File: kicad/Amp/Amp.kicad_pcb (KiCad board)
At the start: 2 copper layers, 30 x 25.6 mm, 31 parts, among them J1 Conn, J2 Conn, J3 Conn, J4 Conn, J5 Conn, U1 TS5A3166DBVR, U2 MCP1700

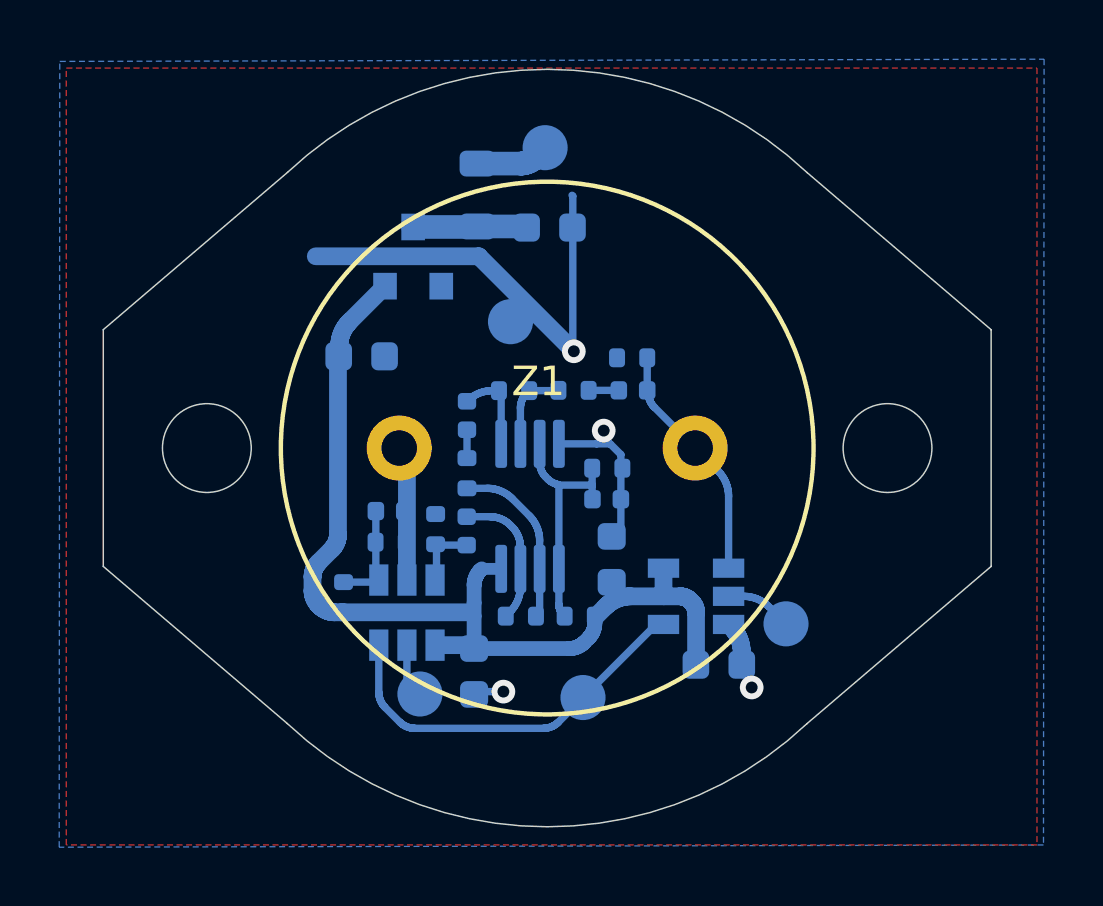
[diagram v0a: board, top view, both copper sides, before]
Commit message: изменено:      kicad/Amp/Amp.kicad_pcb 	изменено:      kicad/Amp/Amp.kicad_pcb-bak 	изменено:      kicad/Amp/Amp.sch 	изменено:      kicad/Amp/Amp.sch-bak 	изменено:      kicad/Amp/fp-info-cache
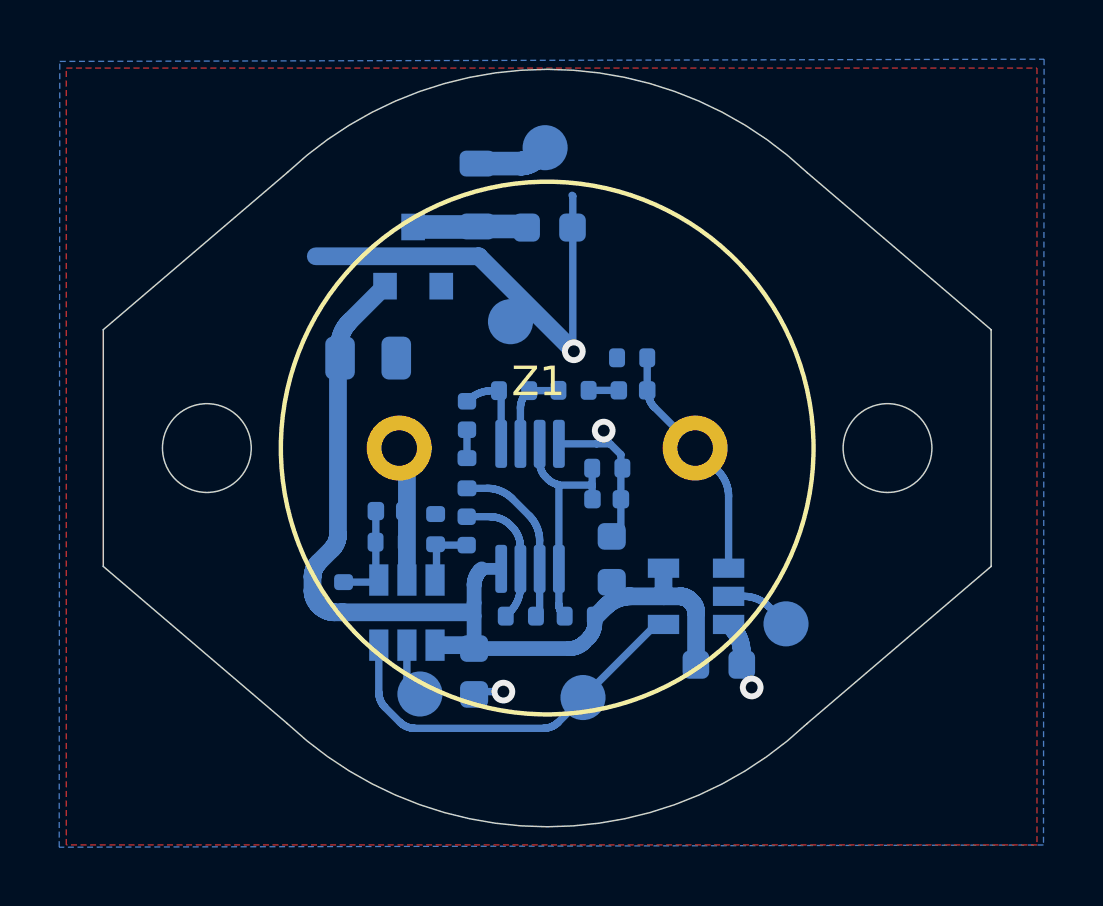
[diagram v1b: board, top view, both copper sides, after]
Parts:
- C5: value .1uF -> 22uF; footprint Capacitor_SMD:C_0603_1608Metric -> Capacitor_SMD:C_0805_2012Metric
- moved C5 0.23 mm to (41.0, 56.2)

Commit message: изменено:      kicad/Amp/Amp.kicad_pcb 	изменено:      kicad/Amp/Amp.kicad_pcb-bak 	изменено:      kicad/Amp/Amp.sch 	изменено:      kicad/Amp/Amp.sch-bak 	изменено:      stm32cubeide/Anemometr_v3/Core/Inc/main.h 	изменено:      stm32cubeide/Anemometr_v3/Core/Src/stm32f1xx_it.c 	изменено:      stm32cubeide/Anemometr_v3/Debug/Anemometr_3.bin 	изменено:      stm32cubeide/Anemometr_v3/Debug/Anemometr_3.elf 	изменено:      stm32cubeide/Anemometr_v3/Debug/Anemometr_3.list 	изменено:      stm32cubeide/Anemometr_v3/Debug/Anemometr_3.map 	изменено:      stm32cubeide/Anemometr_v3/Debug/Core/Src/BME280.o 	изменено:      stm32cubeide/Anemometr_v3/Debug/Core/Src/main.o 	изменено:      stm32cubeide/Anemometr_v3/Debug/Core/Src/main.su 	изменено:      stm32cubeide/Anemometr_v3/Debug/Core/Src/stm32f1xx_hal_msp.o 	изменено:      stm32cubeide/Anemometr_v3/Debug/Core/Src/stm32f1xx_it.o
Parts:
- C7: value 0.1uF -> 2.2uF
